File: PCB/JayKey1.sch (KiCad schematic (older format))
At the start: 24 parts, among them J1 USB_C_Receptacle, J2 USB_C_Receptacle, SW1 SW_PUSH, U1 AT90USB1286, Y1 16M

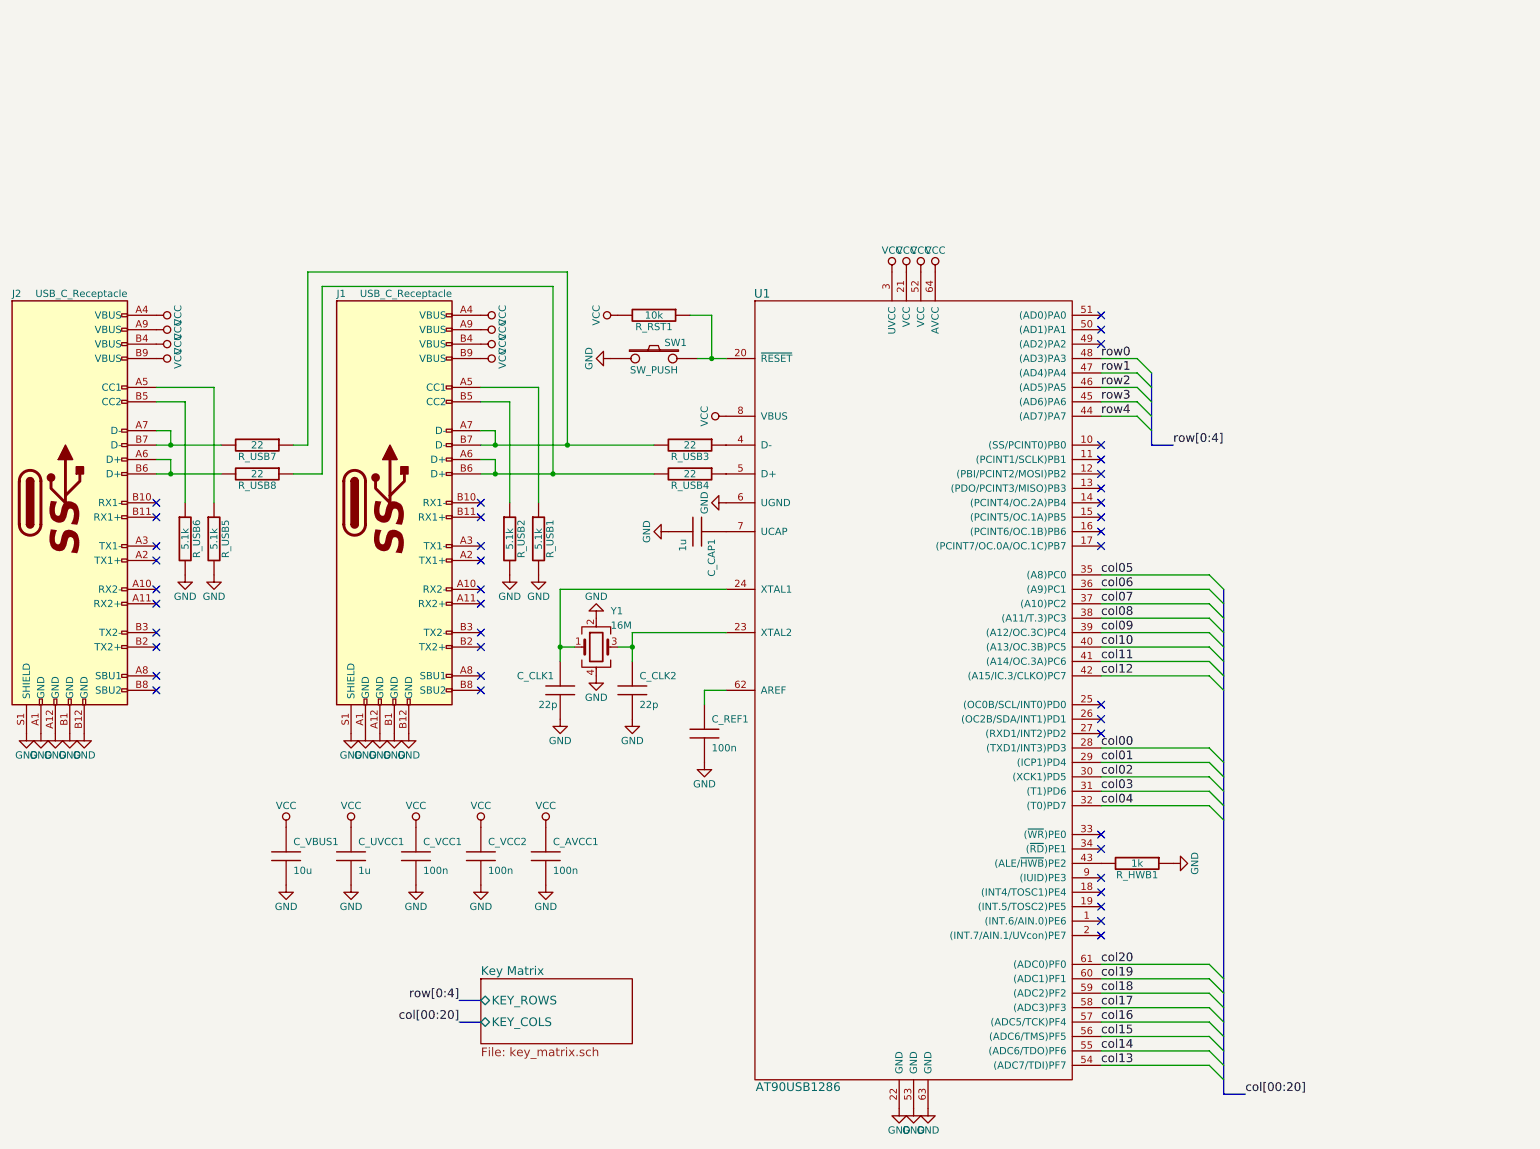
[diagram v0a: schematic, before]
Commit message: 2018.08.28 Nightly
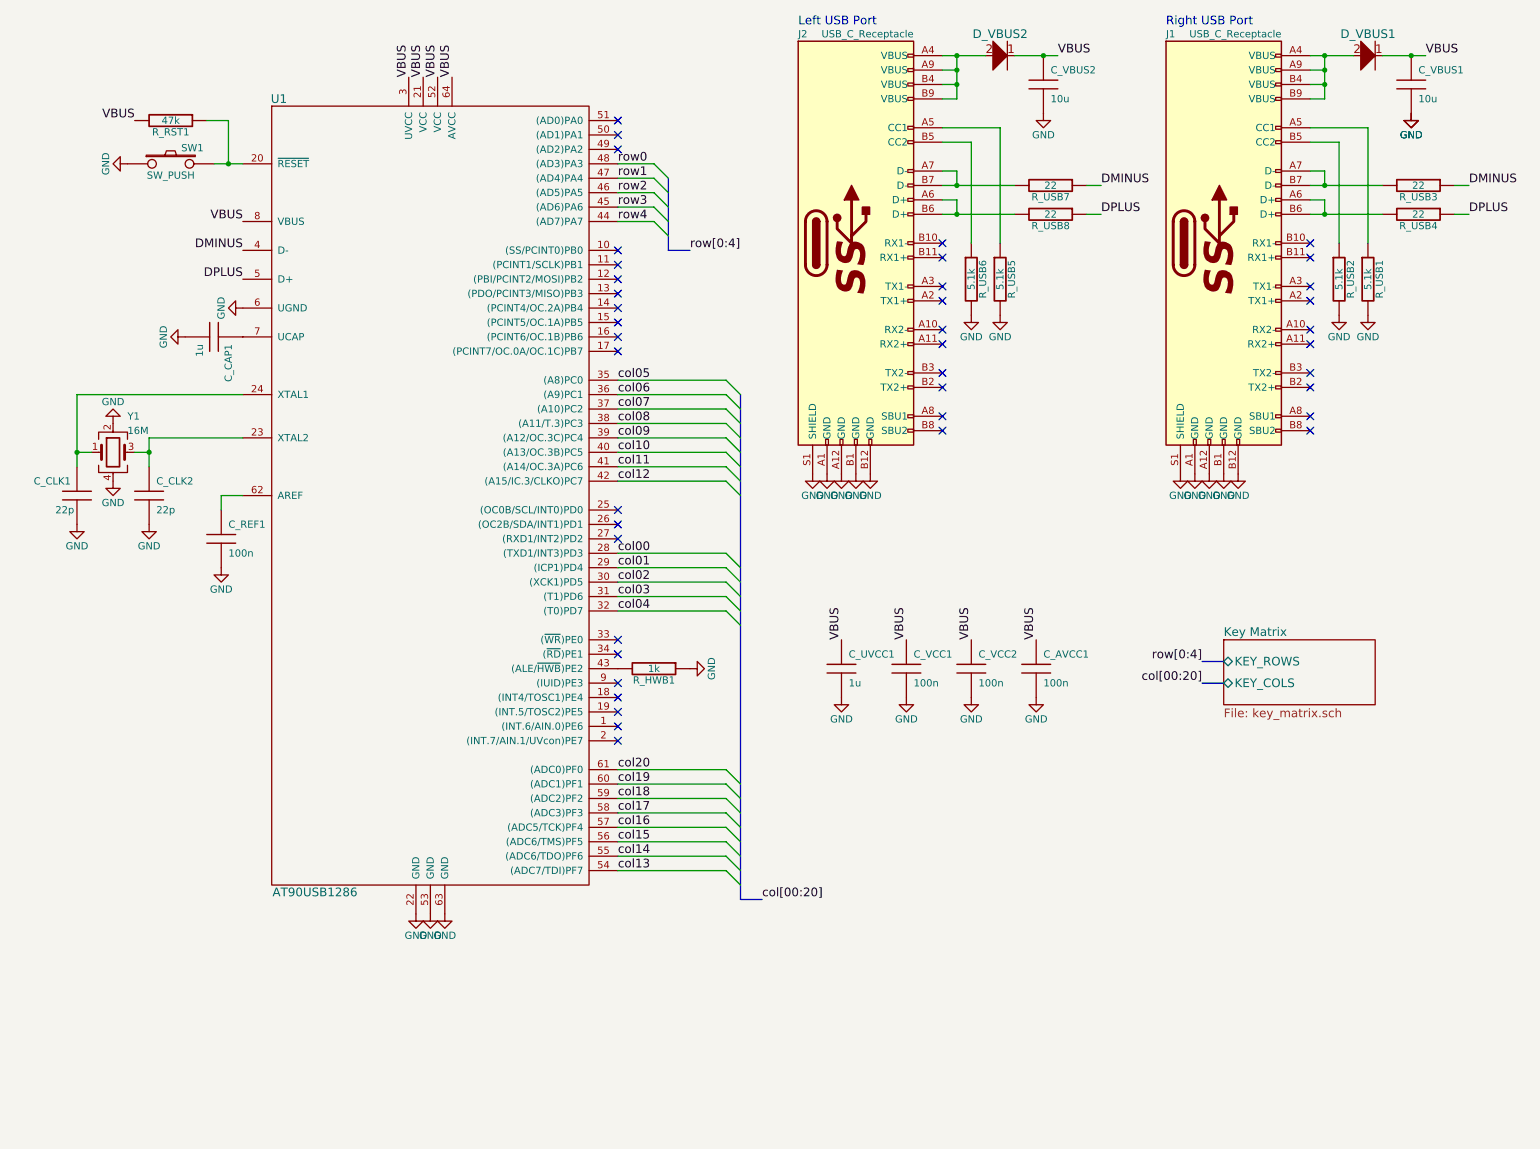
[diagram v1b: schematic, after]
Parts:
- added C_VBUS2: 10u, Capacitors_SMD:C_0805_HandSoldering, symbol C
- added D_VBUS1, D_VBUS2: D, keyboard_parts:D_SOD123_axial, symbol D
- R_RST1: value 10k -> 47k
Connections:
- net GND: now also C_VBUS2.2
- net DMINUS: now reaches R_USB3.1, U1.4 (D-)
- net DMINUS: now also R_USB7.1
- net DPLUS: now reaches R_USB4.1, U1.5 (D+)
- net DPLUS: now also R_USB8.1
- net at J1.A6 (D+), J1.B6 (D+), R_USB4.2: no longer R_USB8.1
- net at J1.A7 (D-), J1.B7 (D-), R_USB3.2: no longer R_USB7.1
- net VCC renamed VBUS
- net VBUS: now also C_VBUS2.1, D_VBUS1.1, D_VBUS2.1; no longer J1.A4 (VBUS), J1.A9 (VBUS), J1.B4 (VBUS), J1.B9 (VBUS), J2.A4 (VBUS), J2.A9 (VBUS), J2.B4 (VBUS), J2.B9 (VBUS)
- new net: D_VBUS1.2, J1.A4 (VBUS), J1.A9 (VBUS), J1.B4 (VBUS), J1.B9 (VBUS)
- new net: D_VBUS2.2, J2.A4 (VBUS), J2.A9 (VBUS), J2.B4 (VBUS), J2.B9 (VBUS)
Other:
- note added: "Left USB Port"
- note added: "Right USB Port"
- moved on the sheet: C_AVCC1, C_CAP1, C_CLK1, C_CLK2, C_REF1, C_UVCC1, C_VCC1, C_VCC2, J1, J2, R_HWB1, R_RST1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

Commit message: 2018.09.23 Nightly
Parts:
- removed C_VBUS1, C_VBUS2: 10u, Capacitors_SMD:C_0805_HandSoldering, symbol C
- removed D_VBUS1, D_VBUS2: D, keyboard_parts:D_SOD123_axial, symbol D
- removed J1, J2: USB_C_Receptacle, Connectors_USB:USB_C_Receptacle_Amphenol_12401610E4-2A, symbol USB_C_Receptacle
- removed R_USB1, R_USB2, R_USB5, R_USB6: 5.1k, Resistors_SMD:R_0805_HandSoldering, symbol R
- removed R_USB3, R_USB4, R_USB7, R_USB8: 22, Resistors_SMD:R_0805_HandSoldering, symbol R
- removed U1: AT90USB1286, Housings_QFP:TQFP-64_14x14mm_Pitch0.8mm, symbol AT90USB1286
- added U1: AT90USB1286-AU, Housings_QFP:TQFP-64_14x14mm_Pitch0.8mm, symbol AT90USB1286-AU
- renumbered C_REF1 to C_AREF1, C_CAP1 to C_UCAP1
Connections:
- wire segments 73 -> 41
- no-connect marks 41 -> 21
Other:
- note removed: "Left USB Port"
- note removed: "Right USB Port"
- moved on the sheet: C_AREF1, C_AVCC1, C_CLK1, C_CLK2, C_UCAP1, C_UVCC1, C_VCC1, C_VCC2, R_HWB1, R_RST1, SW1, Y1
